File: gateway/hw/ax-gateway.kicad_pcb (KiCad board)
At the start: 2 copper layers, 65 x 56 mm, 90 parts, among them IC1 TG-5006CJ, IC2 TPS73433, IC3 AX5243, IC4 AX5243, P1 Raspberry_Pi_Conn, P2 COAX, P3 COAX, P4 PAD

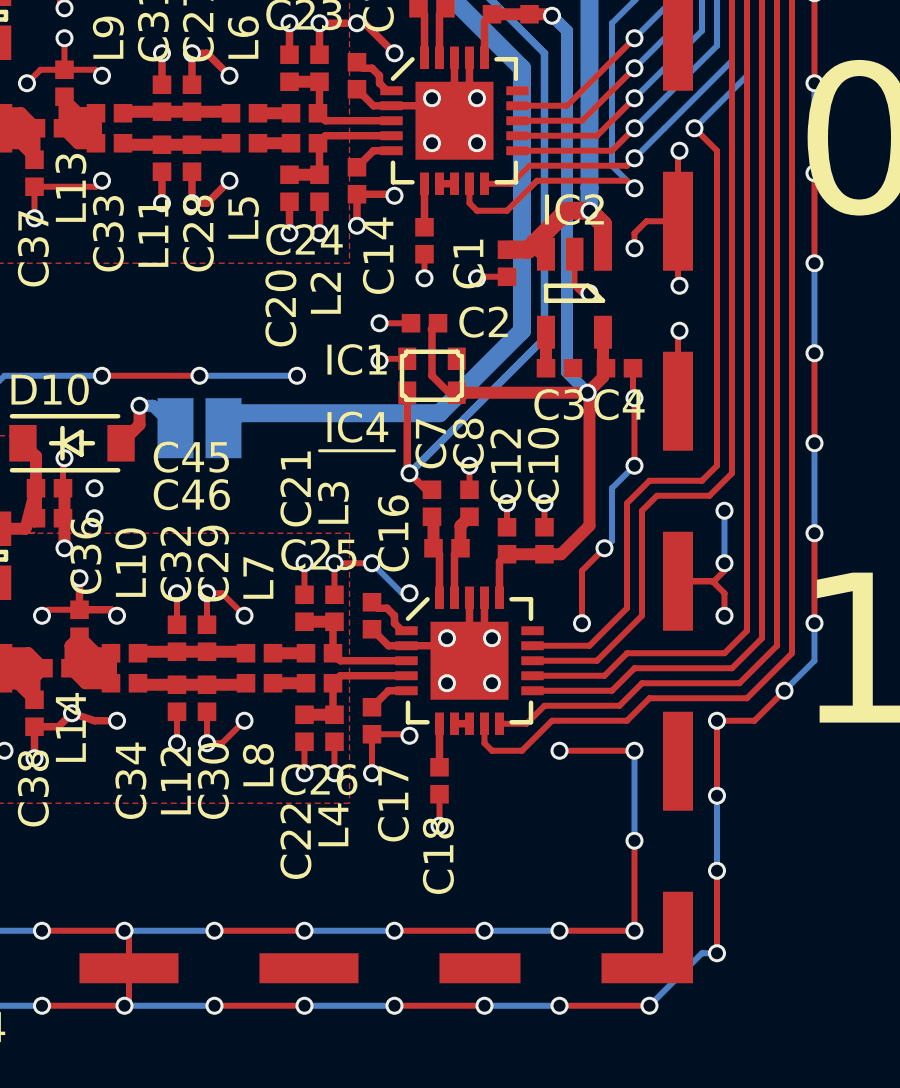
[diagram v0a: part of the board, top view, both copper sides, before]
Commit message: [hw] add l_ext
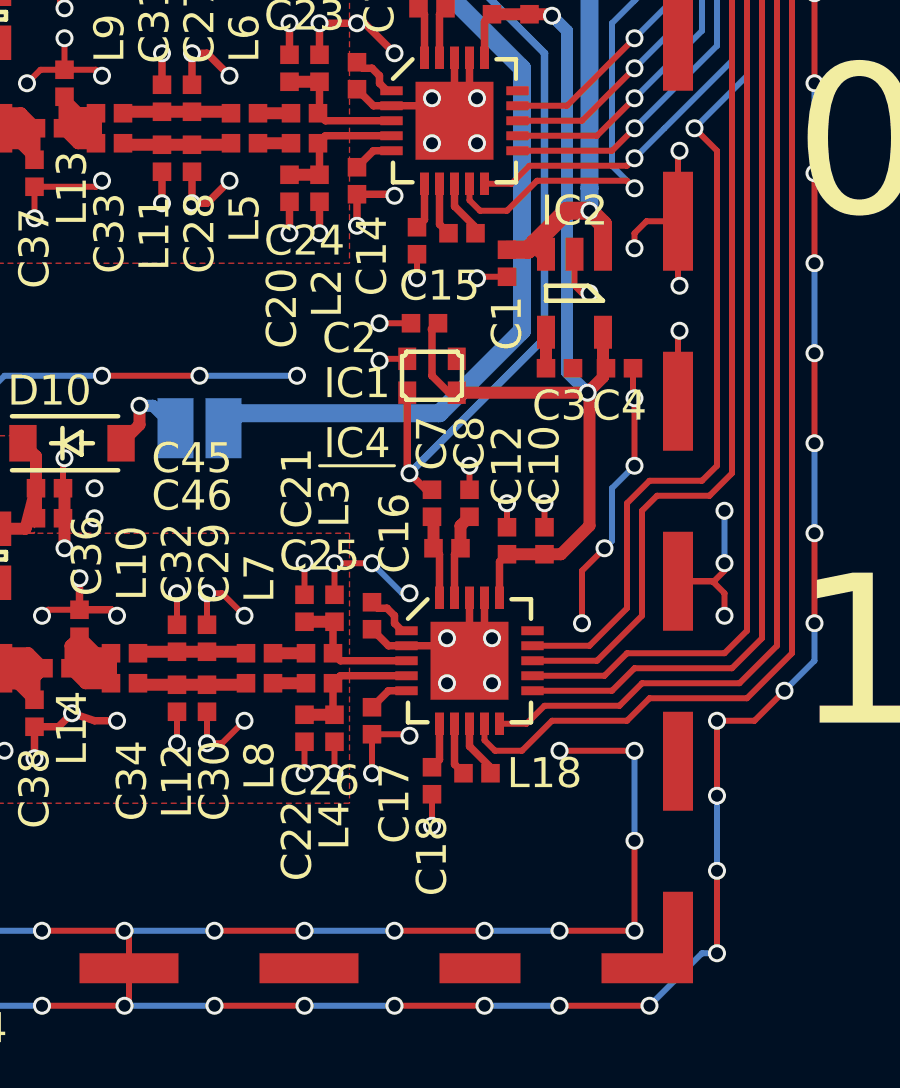
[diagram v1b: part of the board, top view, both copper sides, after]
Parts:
- added L17: 0Ω, agg:0402, F.Cu at (171.8, 108.0)
- added L18: 0Ω, agg:0402, F.Cu at (172.2, 126.0)
- moved C15 0.25 mm to (170.2, 108.2)
- moved C18 0.25 mm to (170.8, 126.2)
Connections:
- IC3 pad 7: /SYNTH_LOOP_0 -> /L1_0
- IC3 pad 8: /SYNTH_LOOP_0 -> /L2_0
- IC4 pad 7: /SYNTH_LOOP_1 -> /L1_1
- IC4 pad 8: /SYNTH_LOOP_1 -> /L2_1
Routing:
- net /L2_1: track 0.00 -> 1.94 mm
- net /L2_0: track 0.00 -> 1.94 mm
- net /L1_1: track 0.00 -> 1.77 mm
- net /L1_0: track 0.00 -> 1.77 mm
- net /SYNTH_LOOP_1: track 0.50 -> 0.00 mm
- net /SYNTH_LOOP_0: track 0.50 -> 0.00 mm
